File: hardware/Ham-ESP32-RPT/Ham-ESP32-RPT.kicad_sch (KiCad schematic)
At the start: 9 parts, among them J5 Conn_01x04_Socket, Q1 MMBT3904, SW1 REP TEST, U4 ESP32-S3-DevKitC

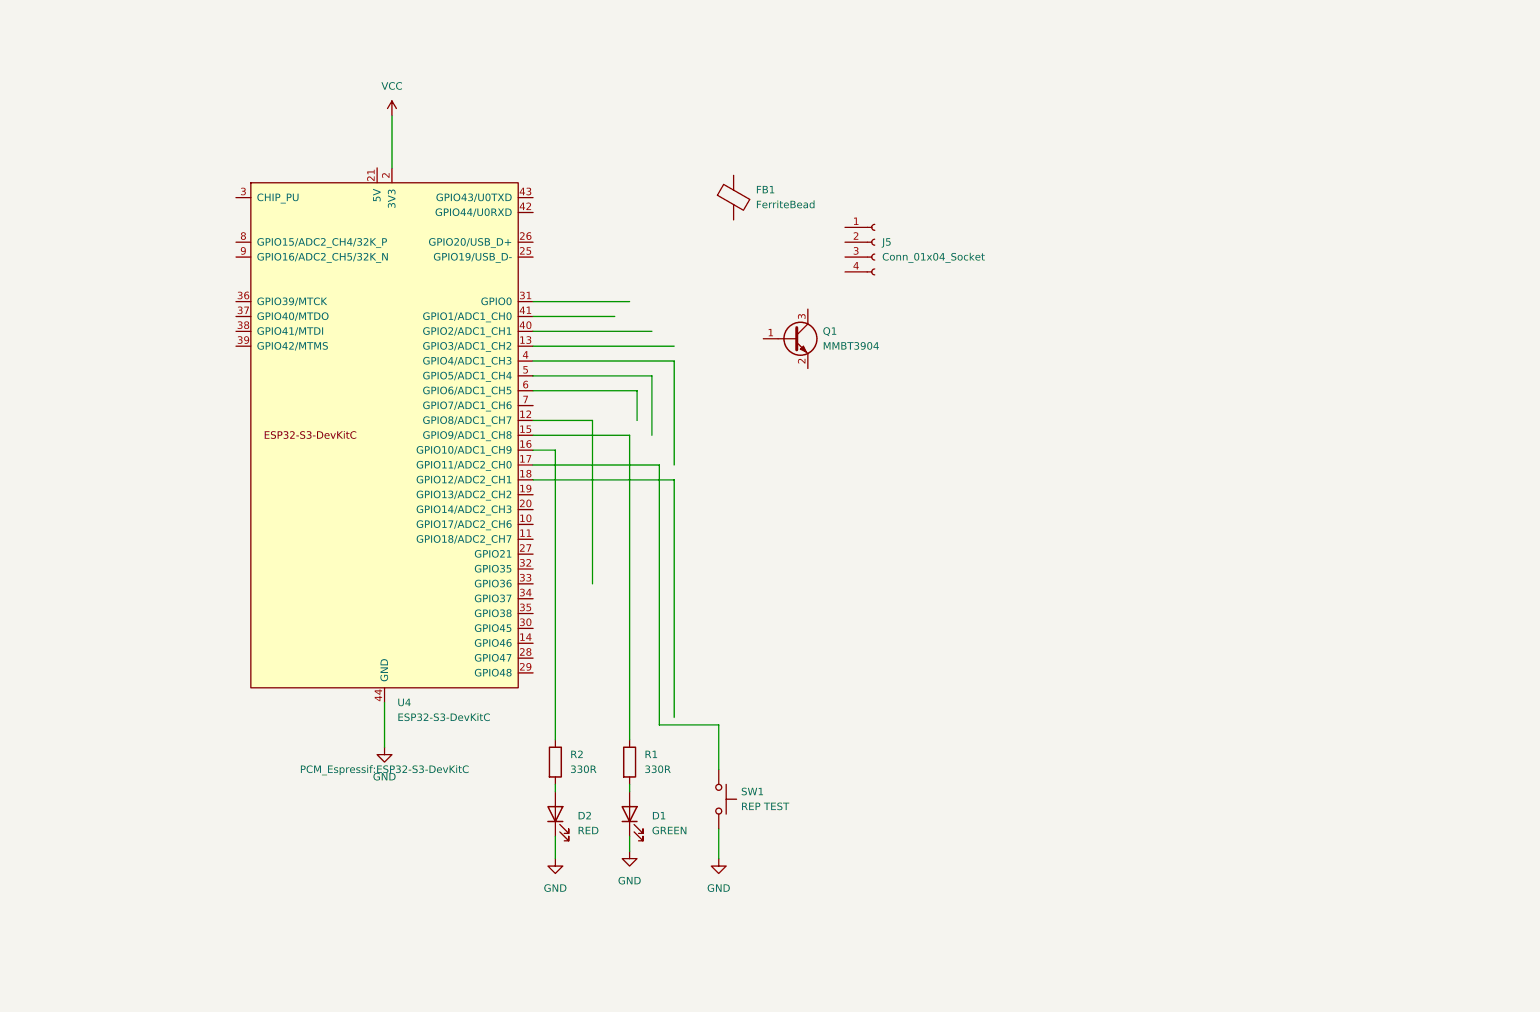
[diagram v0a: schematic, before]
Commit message: PCB kicad update
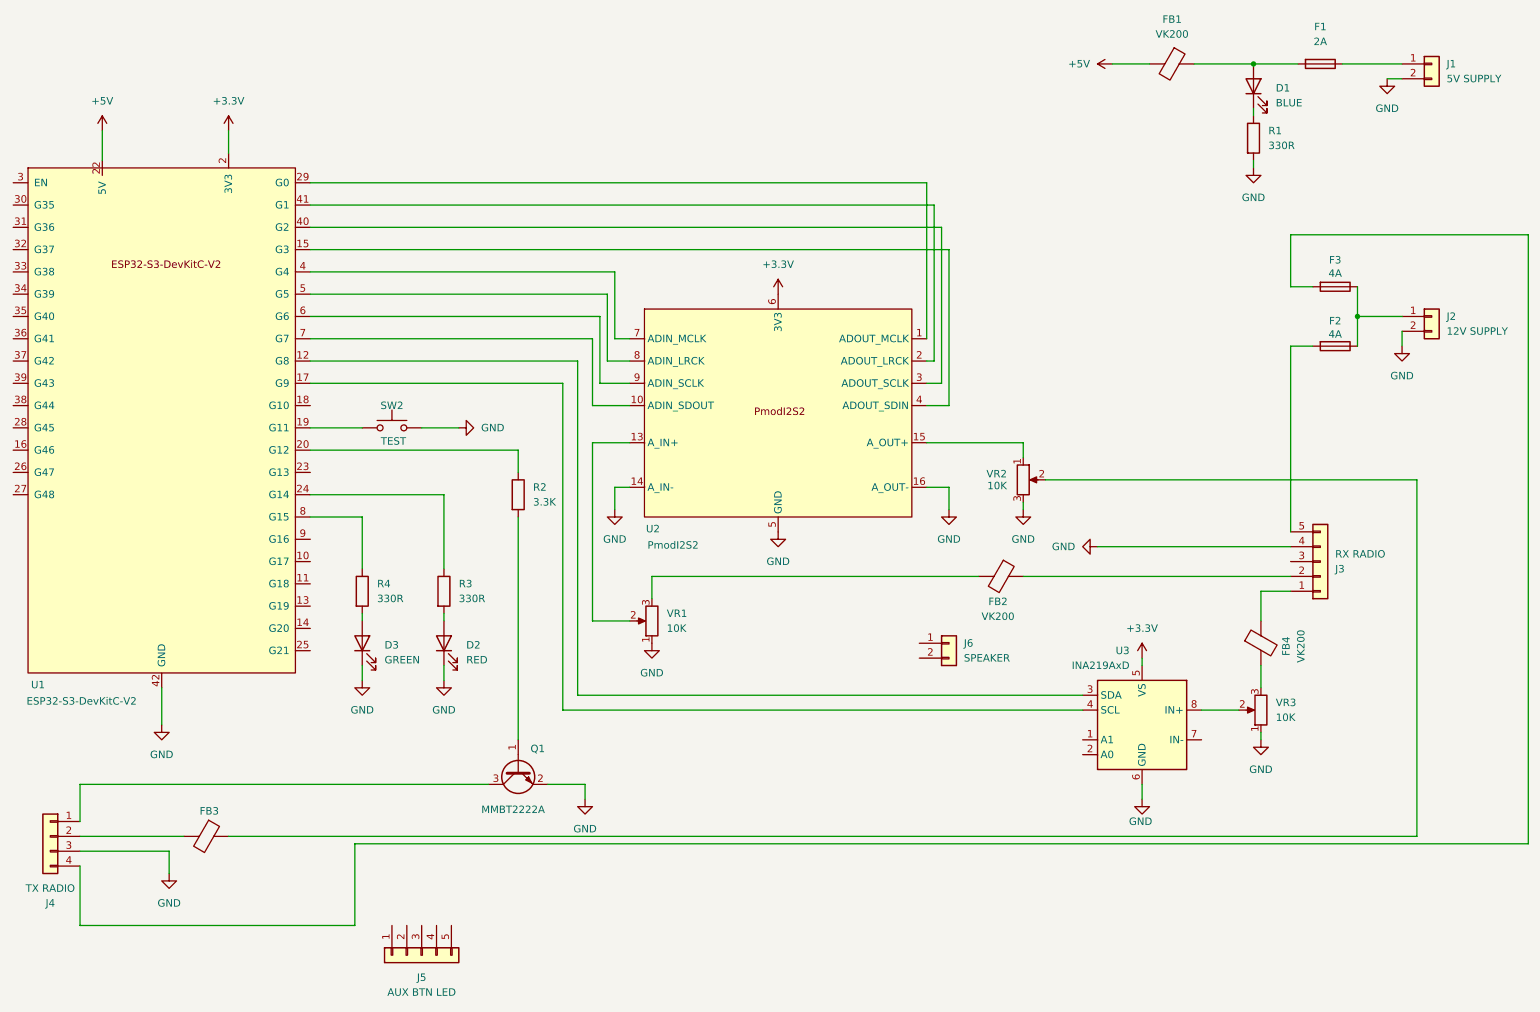
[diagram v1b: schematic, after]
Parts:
- removed J5: Conn_01x04_Socket, Connector_JST:JST_XH_B4B-XH-A_1x04_P2.50mm_Vertical, symbol Connector:Conn_01x04_Socket
- removed Q1: MMBT3904, Package_TO_SOT_SMD:SOT-23, symbol Transistor_BJT:MMBT3904
- removed SW1: REP TEST, Button_Switch_THT:SW_PUSH_6mm, symbol Switch:SW_Push
- removed U4: ESP32-S3-DevKitC, PCM_Espressif:ESP32-S3-DevKitC, symbol PCM_Espressif:ESP32-S3-DevKitC
- added D1: BLUE, LED_SMD:LED_1206_3216Metric, symbol Device:LED
- added F1: 2A, Fuse:Fuse_1206_3216Metric, symbol Device:Fuse
- added F2, F3: 4A, Fuse:Fuse_1206_3216Metric, symbol Device:Fuse
- added FB2, FB3, FB4: VK200, Inductor_SMD:L_Neosid_MicroCoil_Ms36-L, symbol Device:FerriteBead
- added J1: 5V SUPPLY, Connector_JST:JST_XH_B2B-XH-A_1x02_P2.50mm_Vertical, symbol Connector_Generic:Conn_01x02
- added J2: 12V SUPPLY, Connector_JST:JST_XH_B2B-XH-A_1x02_P2.50mm_Vertical, symbol Connector_Generic:Conn_01x02
- added J3: RX RADIO, Connector_JST:JST_XH_B5B-XH-A_1x05_P2.50mm_Vertical, symbol Connector_Generic:Conn_01x05
- added J4: TX RADIO, Connector_JST:JST_XH_B4B-XH-A_1x04_P2.50mm_Vertical, symbol Connector_Generic:Conn_01x04
- added J5: AUX BTN LED, Connector_JST:JST_XH_B5B-XH-A_1x05_P2.50mm_Vertical, symbol Connector_Generic:Conn_01x05
- added J6: SPEAKER, Connector_JST:JST_XH_B2B-XH-A_1x02_P2.50mm_Vertical, symbol Connector_Generic:Conn_01x02
- added Q1: MMBT2222A, Package_TO_SOT_SMD:TSOT-23, symbol Transistor_BJT:MMBT2222A
- added R1: 330R, Resistor_SMD:R_1206_3216Metric, symbol Device:R
- added R2: 3.3K, Resistor_SMD:R_1206_3216Metric, symbol Device:R
- added SW2: TEST, Button_Switch_SMD:SW_Push_1P1T_NO_E-Switch_TL3301NxxxxxG, symbol Switch:SW_Push
- added U1: ESP32-S3-DevKitC-V2, Ham-ESP32-RPT-pretty:ESP32-S3-DevKitC-V2, symbol Ham-ESP32-RPT:ESP32-S3-DevKitC-V2
- added U2: PmodI2S2, symbol Ham-ESP32-RPT:PmodI2S2
- added U3: INA219AxD, Package_SO:SOIC-8_3.9x4.9mm_P1.27mm, symbol Sensor_Energy:INA219AxD
- added VR1, VR2, VR3: 10K, Potentiometer_SMD:Potentiometer_Bourns_3314R-1_Vertical_Hole, symbol Device:R_Potentiometer
- FB1: value FerriteBead -> VK200; footprint Ferrite_THT:LairdTech_28C0236-0JW-10 -> Inductor_SMD:L_Neosid_MicroCoil_Ms36-L
- renumbered D1 to D3, R2 to R3, R1 to R4
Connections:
- net GND: now also J1.2 (Pin_2), J2.2 (Pin_2), J3.4 (Pin_4), J4.3 (Pin_3), Q1.2 (E), R1.2, SW2.2, U1.1 (GND), U1.42 (GND), U2.11 (GND), U2.14 (A_IN-), U2.16 (A_OUT-), U2.5 (GND), U3.6 (GND), VR1.1, VR2.3, VR3.1
- net at R4.1: now also U1.8 (G15)
- net at R3.1: now also U1.24 (G14)
- net at FB1.1: now also D1.2 (A), F1.2
- net +5V: now reaches FB1.2
- net +5V: now also U1.22 (5V)
- new net: R2.1, U1.20 (G12)
- new net: Q1.1 (B), R2.2
- new net: U2.13 (A_IN+), VR1.2
- new net: FB2.2, VR1.3
- new net: D1.1 (K), R1.1
- new net: FB4.1, J3.1 (Pin_1)
- new net: FB2.1, J3.2 (Pin_2)
- new net: F2.2, J3.5 (Pin_5)
- new net: F1.1, J1.1 (Pin_1)
- new net: U1.12 (G8), U3.3 (SDA)
- new net: U1.15 (G3), U2.4 (ADOUT_SDIN)
- new net: U1.17 (G9), U3.4 (SCL)
- new net: SW2.1, U1.19 (G11)
- new net: U1.29 (G0), U2.1 (ADOUT_MCLK)
- new net: U1.4 (G4), U2.7 (ADIN_MCLK)
- new net: U1.40 (G2), U2.3 (ADOUT_SCLK)
- new net: U1.41 (G1), U2.2 (ADOUT_LRCK)
- new net: U1.5 (G5), U2.8 (ADIN_LRCK)
- new net: U1.6 (G6), U2.9 (ADIN_SCLK)
- new net: U1.7 (G7), U2.10 (ADIN_SDOUT)
- new net: J4.1 (Pin_1), Q1.3 (C)
- new net: FB3.2, J4.2 (Pin_2)
- new net: F3.2, J4.4 (Pin_4)
- new net: U2.15 (A_OUT+), VR2.1
- new net: FB4.2, VR3.3
- new net: FB3.1, VR2.2
- new net: F2.1, F3.1, J2.1 (Pin_1)
- new net: U3.8 (IN+), VR3.2
- new net +3.3V: U1.2 (3V3), U1.21 (3V3), U2.12 (3V3), U2.6 (3V3), U3.5 (VS)
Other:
- moved on the sheet: D2, D3, FB1, R3, R4
